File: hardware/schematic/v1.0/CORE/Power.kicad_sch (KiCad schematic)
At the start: 11 parts, among them U2 TPS78633, U5 AMS1117-1.8

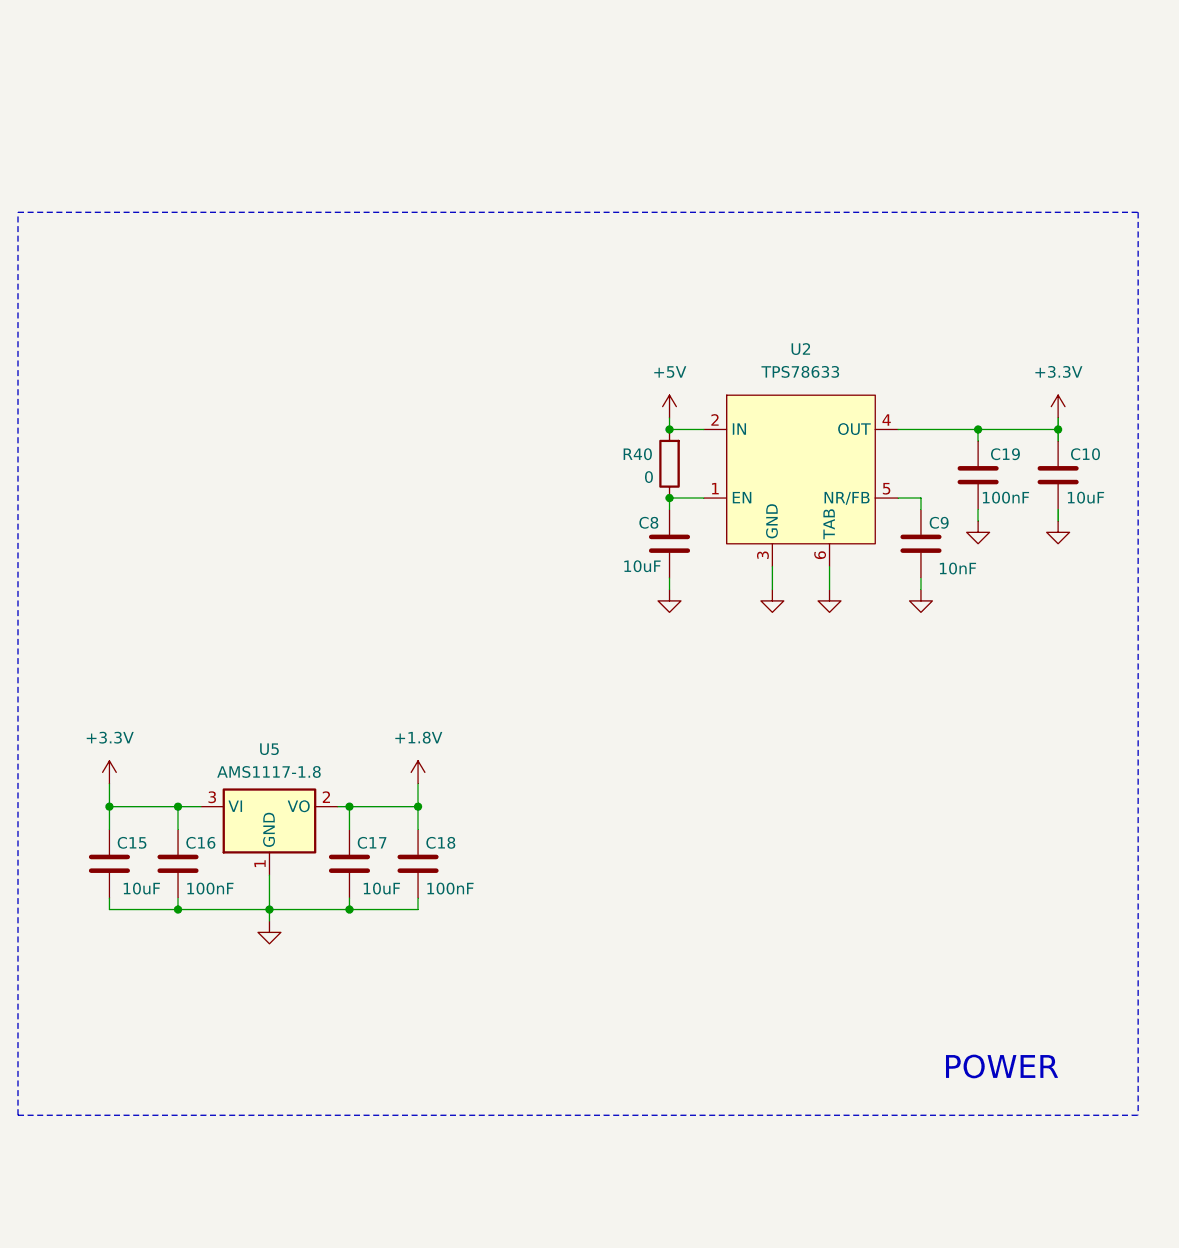
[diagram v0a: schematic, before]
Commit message: sch update
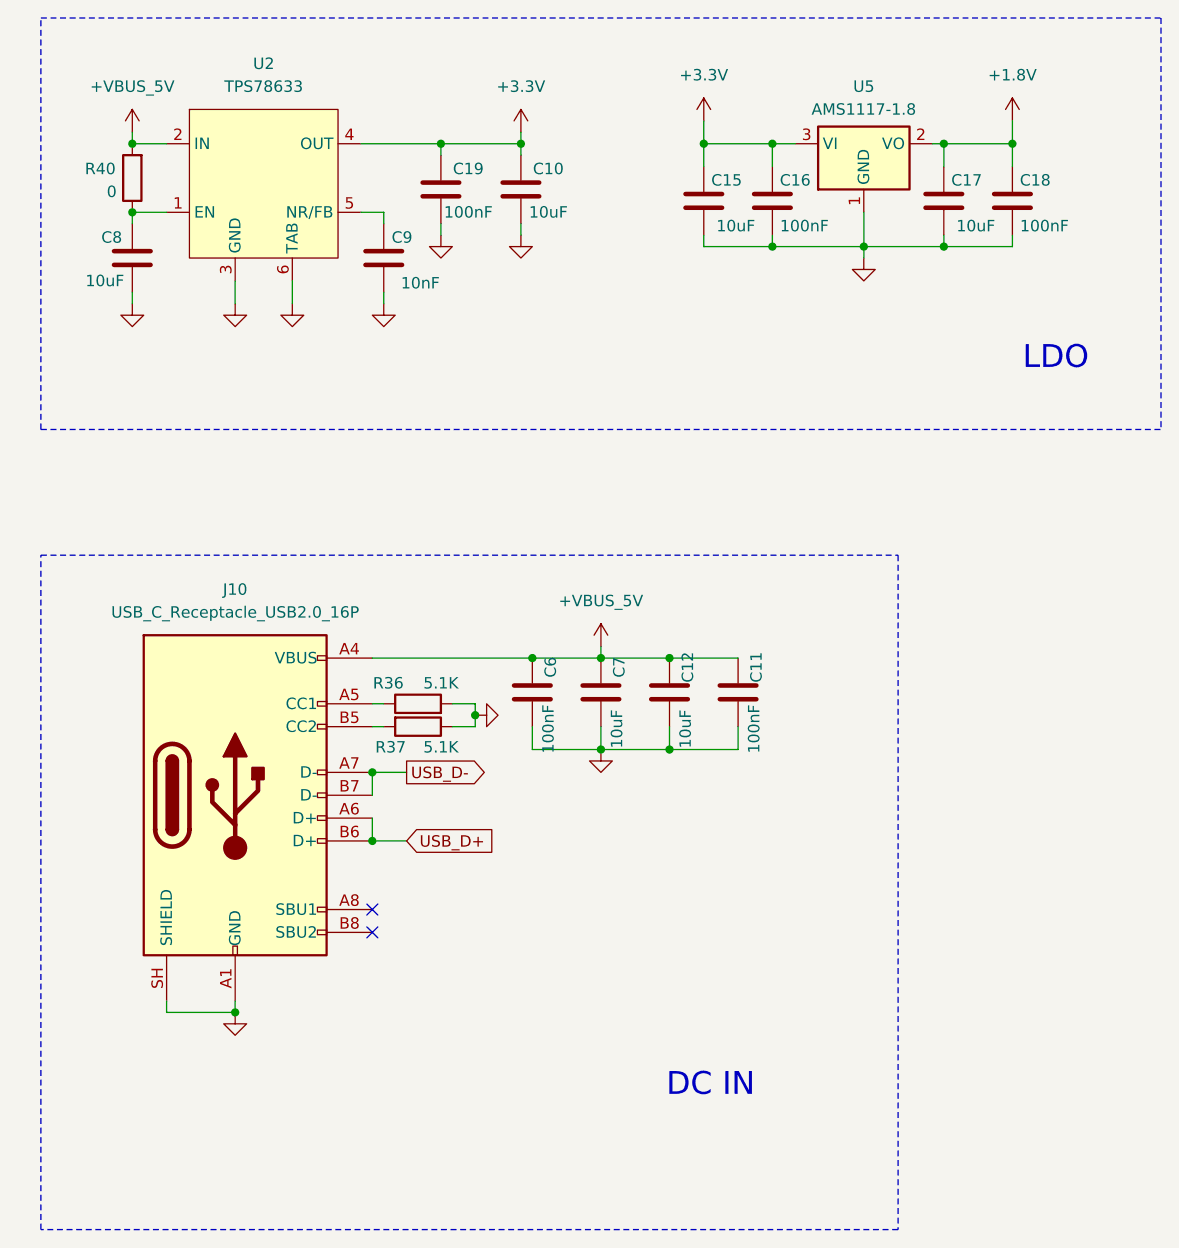
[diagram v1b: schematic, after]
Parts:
- added C11, C6: 100nF, Capacitor_SMD:C_0402_1005Metric, symbol Device:C
- added C12, C7: 10uF, Capacitor_SMD:C_0603_1608Metric, symbol Device:C
- added J10: USB_C_Receptacle_USB2.0_16P, Connector_USB:USB_C_Receptacle_Palconn_UTC16-G, symbol Connector:USB_C_Receptacle_USB2.0_16P
- added R36, R37: 5.1K, Resistor_SMD:R_0402_1005Metric, symbol Device:R
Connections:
- net GND: now also C11.2, C12.2, C6.2, C7.2, J10.A1 (GND), J10.A12 (GND), J10.B1 (GND), J10.B12 (GND), J10.SH (SHIELD), R36.2, R37.1
- net +5V renamed +VBUS_5V
- net +VBUS_5V: now also C11.1, C12.1, C6.1, C7.1, J10.A4 (VBUS), J10.A9 (VBUS), J10.B4 (VBUS), J10.B9 (VBUS)
- new net: J10.A5 (CC1), R36.1
- new net: J10.B5 (CC2), R37.2
- new net USB_D+: J10.A6 (D+), J10.B6 (D+)
- new net USB_D-: J10.A7 (D-), J10.B7 (D-)
- no-connect marks 0 -> 2
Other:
- note added: "DC IN"
- note added: "LDO"
- note removed: "POWER"
- moved on the sheet: C10, C15, C16, C17, C18, C19, C8, C9, R40, U2, U5
